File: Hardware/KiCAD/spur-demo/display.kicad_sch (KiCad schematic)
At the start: 6 parts

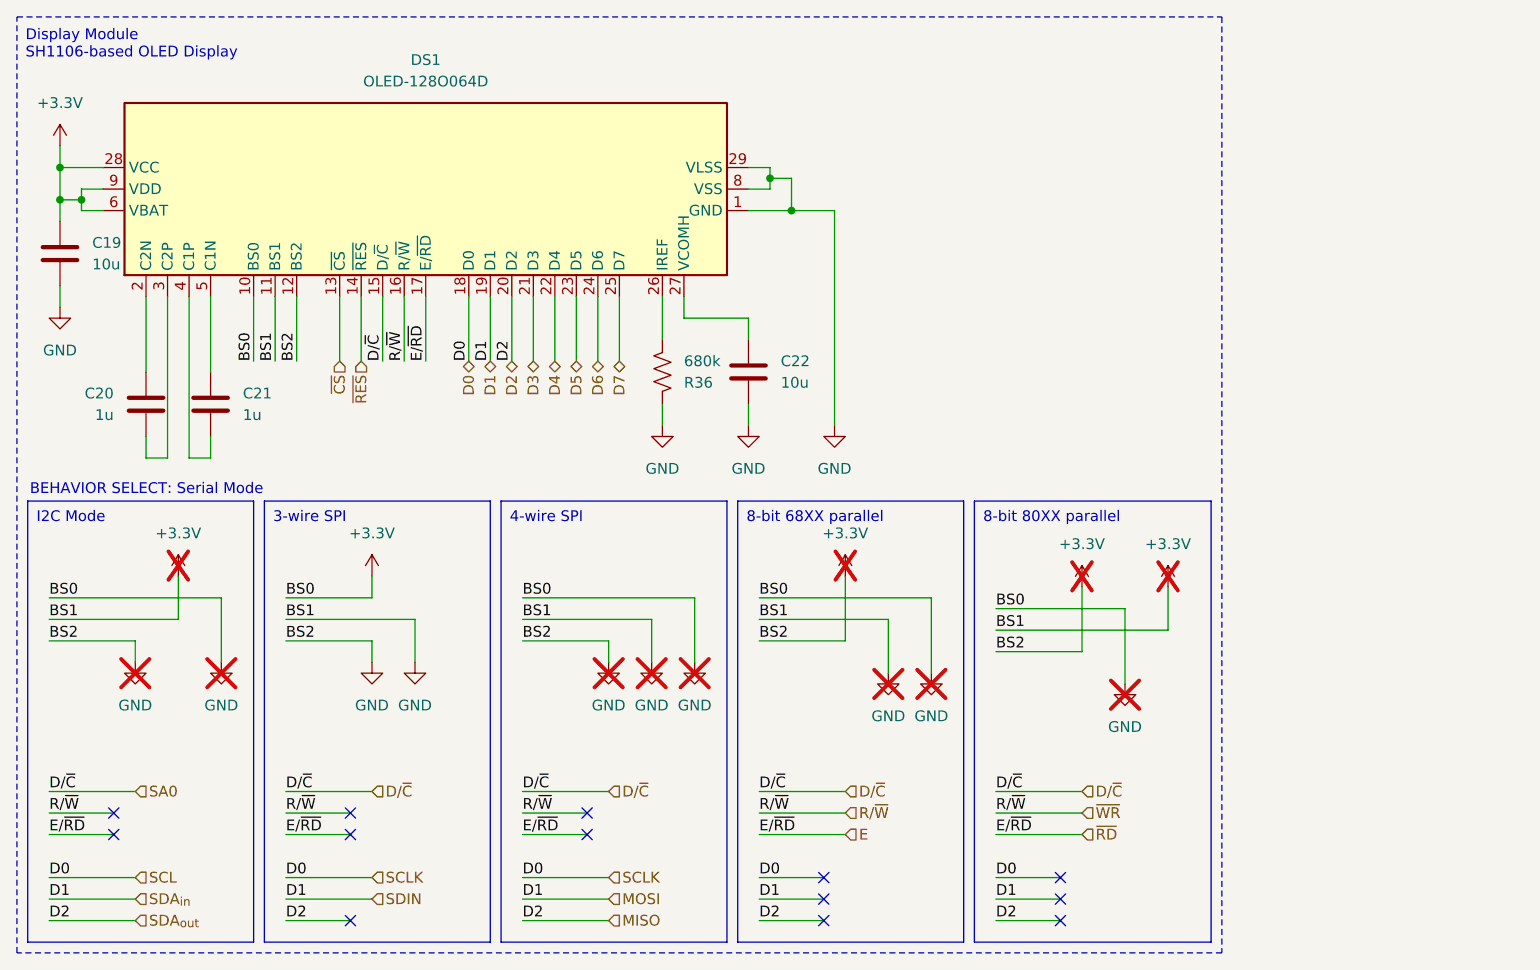
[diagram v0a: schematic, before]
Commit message: feat: add behavior select solder jumpers: default 3-wire SPI
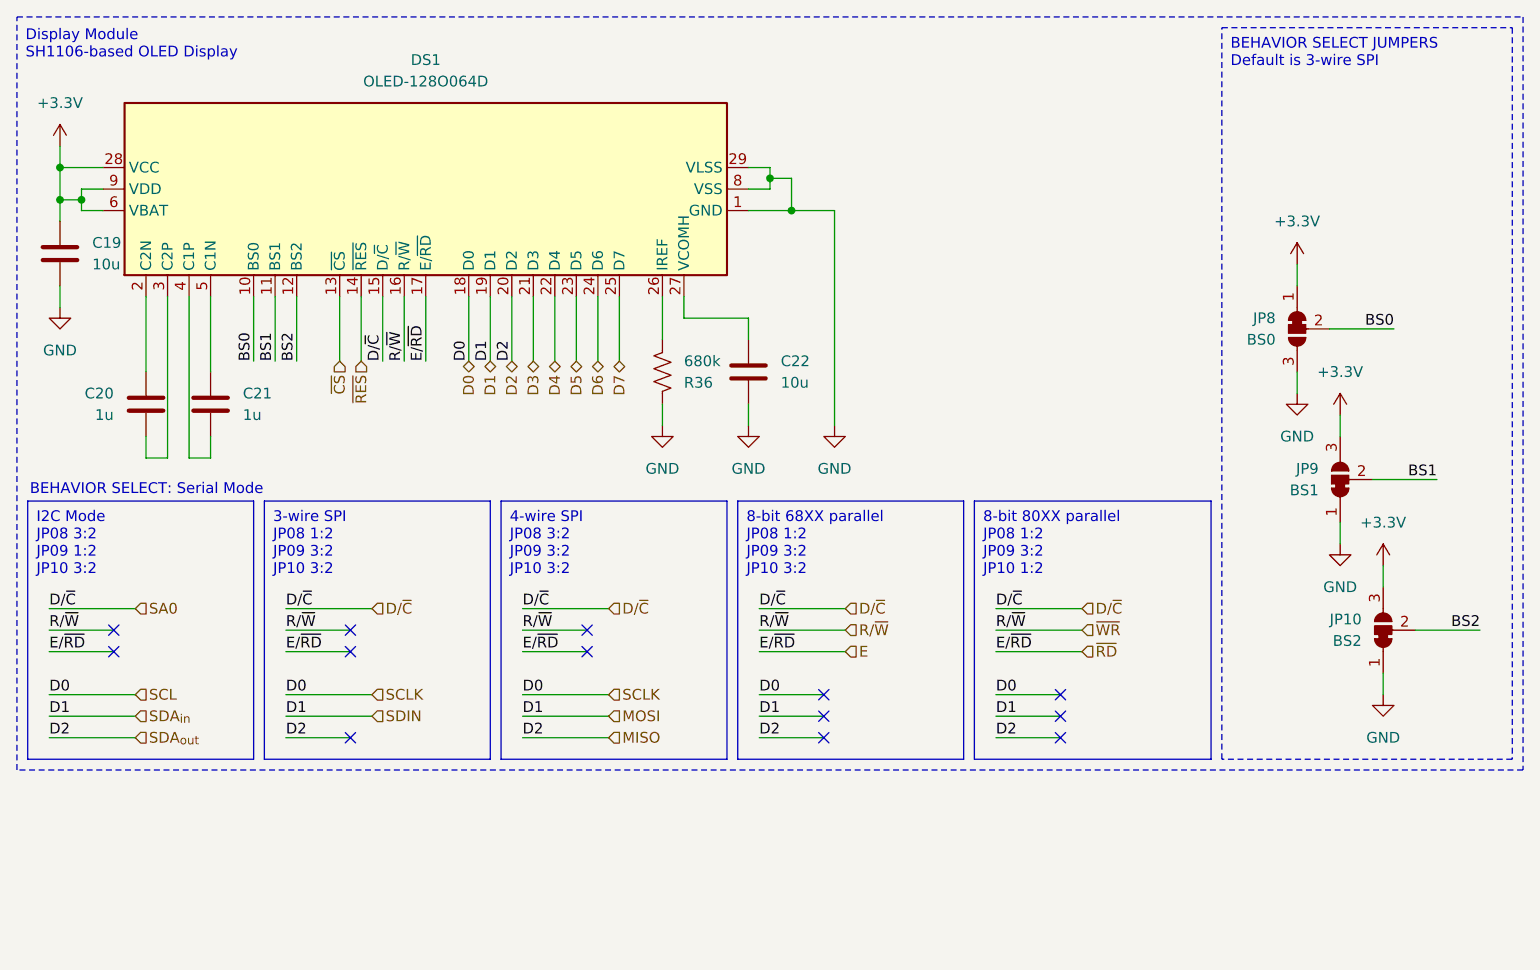
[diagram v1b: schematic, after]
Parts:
- added JP10: BS2, symbol Jumper:SolderJumper_3_Bridged12
- added JP8: BS0, symbol Jumper:SolderJumper_3_Bridged12
- added JP9: BS1, symbol Jumper:SolderJumper_3_Bridged12
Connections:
- net +3.3V: now also JP10.3 (B), JP8.1 (A), JP9.3 (B); no longer C19.2, C22.2, DS1.1 (GND), DS1.10 (BS0), DS1.11 (BS1), DS1.12 (BS2), DS1.29 (VLSS), DS1.30 (GND), DS1.8 (VSS), R36.1
- new net BS0: DS1.10 (BS0), JP8.2 (C)
- new net BS1: DS1.11 (BS1), JP9.2 (C)
- new net BS2: DS1.12 (BS2), JP10.2 (C)
- new net GND: C19.2, C22.2, DS1.1 (GND), DS1.29 (VLSS), DS1.30 (GND), DS1.8 (VSS), JP10.1 (A), JP8.3 (B), JP9.1 (A), R36.1
